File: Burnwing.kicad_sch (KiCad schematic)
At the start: 42 parts, among them J1 USB Type C, J2 Conn_01x06_MountingPin, J4 Conn_01x04_Pin, Q2 AONR21307, SW1 SW_DIP_x02, U1 HUSB238, U2 BTS7030-2EPA

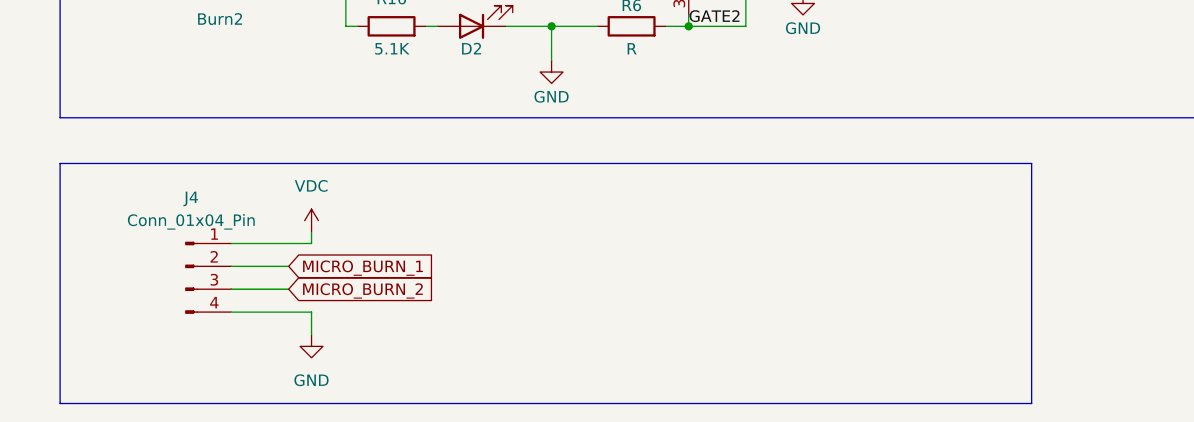
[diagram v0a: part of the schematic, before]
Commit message: Schematic Update
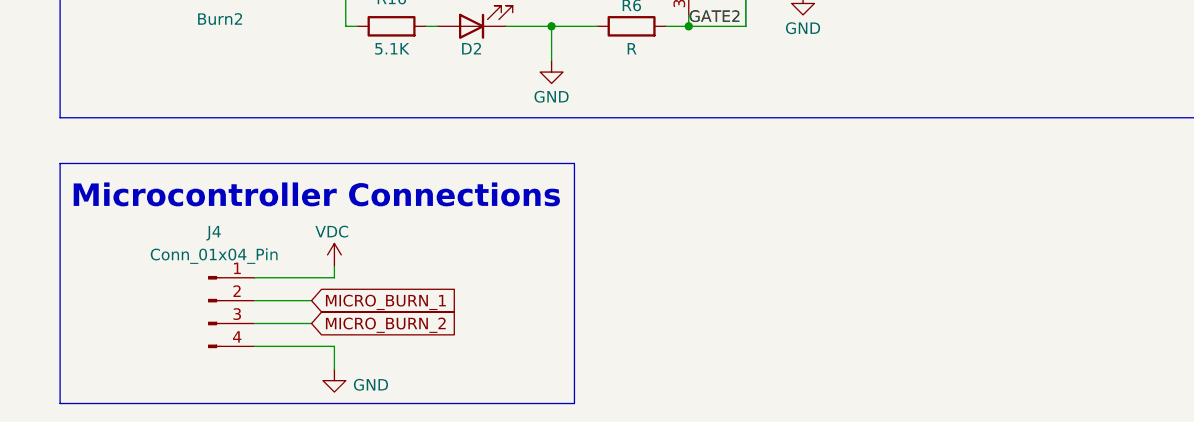
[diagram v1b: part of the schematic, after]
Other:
- note added: "Microcontroller Connections"
- moved on the sheet: J4
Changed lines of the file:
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@@
 	(rectangle
 		(start 17.78 172.72)
-		(end 125.73 199.39)
+		(end 74.93 199.39)
 		(stroke
 			(width 0)
@@
 		)
 	)
+	(text "Microcontroller Connections"
+		(exclude_from_sim no)
+		(at 46.228 176.53 0)
+		(effects
+			(font
+				(size 2.5 2.5)
+				(thickness 0.5)
+				(bold yes)
+			)
+		)
+	)
 	(text "Power LED"
 		(exclude_from_sim no)
@@
 	(wire
 		(pts
-			(xy 36.83 184.15) (xy 43.18 184.15)
+			(xy 39.37 187.96) (xy 45.72 187.96)
 		)
 		(stroke
@@
 	(wire
 		(pts
-			(xy 36.83 186.69) (xy 43.18 186.69)
+			(xy 39.37 190.5) (xy 45.72 190.5)
 		)
 		(stroke
@@
 	(wire
 		(pts
-			(xy 36.83 181.61) (xy 45.72 181.61)
+			(xy 39.37 185.42) (xy 48.26 185.42)
 		)
 		(stroke
@@
 	(wire
 		(pts
-			(xy 45.72 189.23) (xy 45.72 191.77)
+			(xy 48.26 193.04) (xy 48.26 195.58)
 		)
 		(stroke
@@
 	(wire
 		(pts
-			(xy 36.83 189.23) (xy 45.72 189.23)
+			(xy 39.37 193.04) (xy 48.26 193.04)
 		)
 		(stroke
@@
 	(wire
 		(pts
-			(xy 45.72 181.61) (xy 45.72 180.34)
+			(xy 48.26 185.42) (xy 48.26 184.15)
 		)
 		(stroke
@@
 	(global_label "MICRO_BURN_2"
 		(shape input)
-		(at 43.18 186.69 0)
+		(at 45.72 190.5 0)
 		(fields_autoplaced yes)
 		(effects
@@
 		)
 		(property "Intersheetrefs" "${INTERSHEET_REFS}"
-			(at 60.4376 186.69 0)
+			(at 62.9776 190.5 0)
 			(effects
 				(font
@@
 	(global_label "MICRO_BURN_1"
 		(shape input)
-		(at 43.18 184.15 0)
+		(at 45.72 187.96 0)
 		(fields_autoplaced yes)
 		(effects
@@
 		)
 		(property "Intersheetrefs" "${INTERSHEET_REFS}"
-			(at 60.4376 184.15 0)
+			(at 62.9776 187.96 0)
 			(effects
 				(font
@@
 	(symbol
 		(lib_id "power:GND")
-		(at 45.72 191.77 0)
+		(at 48.26 195.58 0)
 		(unit 1)
 		(exclude_from_sim no)
@@
 		(on_board yes)
 		(dnp no)
-		(fields_autoplaced yes)
 		(property "Reference" "#PWR026"
-			(at 45.72 198.12 0)
+			(at 48.26 201.93 0)
 			(effects
 				(font
@@
 		)
 		(property "Value" "GND"
-			(at 45.72 196.85 0)
+			(at 52.324 197.358 0)
 			(effects
 				(font
@@
 		)
 		(property "Footprint" ""
-			(at 45.72 191.77 0)
+			(at 48.26 195.58 0)
 			(effects
 				(font
@@
 		)
 		(property "Datasheet" ""
-			(at 45.72 191.77 0)
+			(at 48.26 195.58 0)
 			(effects
 				(font
@@
 		)
 		(property "Description" "Power symbol creates a global label with name \"GND\" , ground"
-			(at 45.72 191.77 0)
+			(at 48.26 195.58 0)
 			(effects
 				(font
@@
 	(symbol
 		(lib_id "Connector:Conn_01x04_Pin")
-		(at 31.75 184.15 0)
+		(at 34.29 187.96 0)
 		(unit 1)
 		(exclude_from_sim no)
@@
 		(fields_autoplaced yes)
 		(property "Reference" "J4"
-			(at 32.385 176.53 0)
+			(at 34.925 180.34 0)
 			(effects
 				(font
@@
 		)
 		(property "Value" "Conn_01x04_Pin"
-			(at 32.385 179.07 0)
+			(at 34.925 182.88 0)
 			(effects
 				(font
@@
 		)
 		(property "Footprint" "Connector_PinSocket_1.00mm:PinSocket_1x04_P1.00mm_Vertical"
-			(at 31.75 184.15 0)
+			(at 34.29 187.96 0)
 			(effects
 				(font
@@
 		)
 		(property "Datasheet" "~"
-			(at 31.75 184.15 0)
+			(at 34.29 187.96 0)
 			(effects
 				(font
@@
 		)
 		(property "Description" "Generic connector, single row, 01x04, script generated"
-			(at 31.75 184.15 0)
+			(at 34.29 187.96 0)
 			(effects
 				(font
@@
 	(symbol
 		(lib_id "power:VDC")
-		(at 45.72 180.34 0)
+		(at 48.26 184.15 0)
 		(unit 1)
 		(exclude_from_sim no)
@@
 		(on_board yes)
 		(dnp no)
-		(fields_autoplaced yes)
 		(property "Reference" "#PWR025"
-			(at 45.72 184.15 0)
+			(at 48.26 187.96 0)
 			(effects
 				(font
@@
 		)
 		(property "Value" "VDC"
-			(at 45.72 175.26 0)
+			(at 48.006 180.34 0)
 			(effects
 				(font
@@
 		)
 		(property "Footprint" ""
-			(at 45.72 180.34 0)
+			(at 48.26 184.15 0)
 			(effects
 				(font
@@
 		)
 		(property "Datasheet" ""
-			(at 45.72 180.34 0)
+			(at 48.26 184.15 0)
 			(effects
 				(font
@@
 		)
 		(property "Description" "Power symbol creates a global label with name \"VDC\""
-			(at 45.72 180.34 0)
+			(at 48.26 184.15 0)
 			(effects
 				(font
